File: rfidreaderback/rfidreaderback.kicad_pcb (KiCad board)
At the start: 2 copper layers, 85 x 56 mm, 1 part, among them P1 CONN_13X2

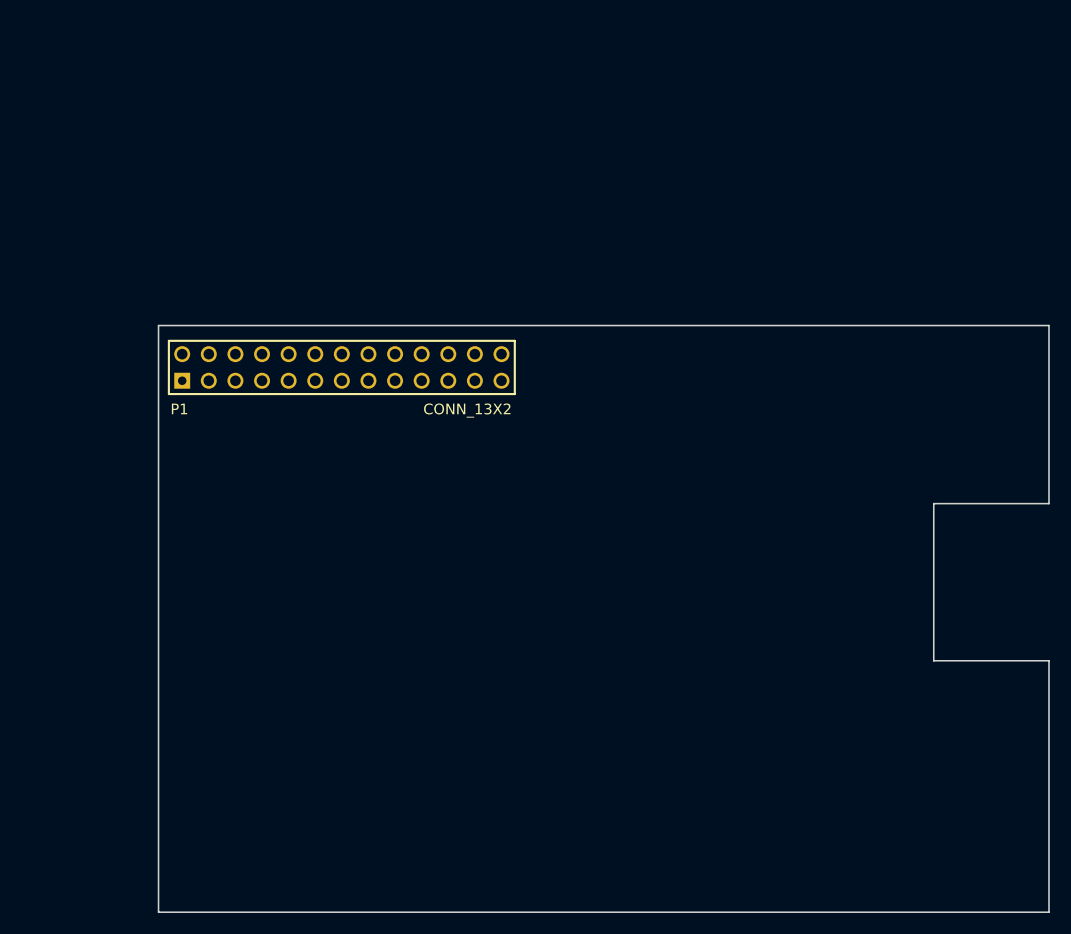
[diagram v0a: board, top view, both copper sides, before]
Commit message: RFID back
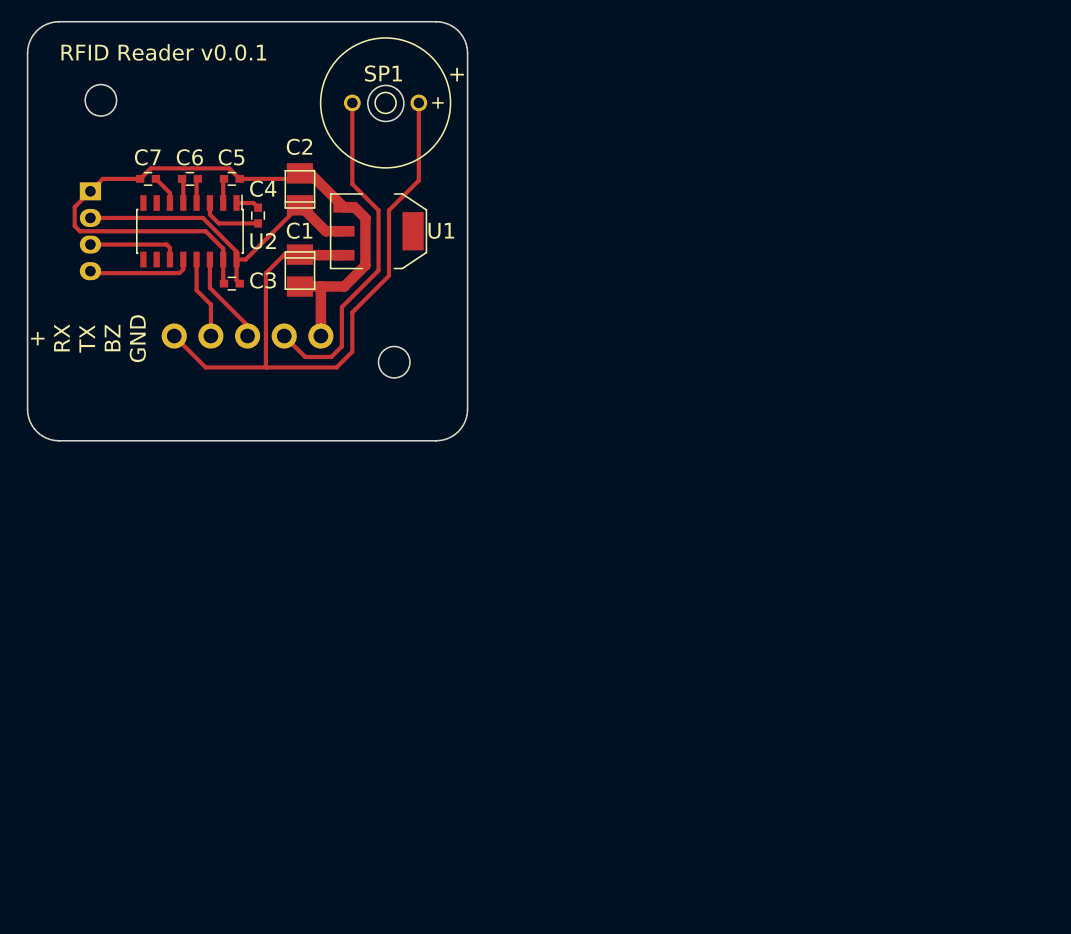
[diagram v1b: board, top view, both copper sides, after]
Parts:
- added C1: 22µ, Capacitors_Tantalum_SMD:TantalC_SizeT_EIA-3528, F.Cu at (157.0, 119.8)
- added C2: 22µ, Capacitors_Tantalum_SMD:TantalC_SizeT_EIA-3528, F.Cu at (157.0, 112.0)
- added C3: 1µ, Capacitors_SMD:C_0603, F.Cu at (150.5, 121.0)
- added C4: 1µ, Capacitors_SMD:C_0603, F.Cu at (153.0, 114.5)
- added C5: 1µ, Capacitors_SMD:C_0603, F.Cu at (150.5, 111.0)
- added C6: 1µ, Capacitors_SMD:C_0603, F.Cu at (146.5, 111.0)
- added C7: 1µ, Capacitors_SMD:C_0603, F.Cu at (142.5, 111.0)
- added P2: PI, pidoor:3_5mm_terminal_1x05, F.Cu at (152.0, 126.0)
- added SP1: MCABI-020-RC, Buzzers_Beepers:MagneticBuzzer_ProSignal_ABT-410-RC, F.Cu at (162.0, 103.8)
- added U1: LD1117S50TR, TO_SOT_Packages_SMD:SOT-223, F.Cu at (164.5, 116.0)
- added U2: ST232BDR, Housings_SOIC:SOIC-16_3.9x9.9mm_Pitch1.27mm, F.Cu at (146.5, 116.0)
- P1: value CONN_13X2 -> READER; footprint pin_array_13x2 -> Socket_Strips:Socket_Strip_Straight_1x04; moved to B.Cu
- moved P1 27.3 mm to (137.0, 116.0), turned to 270 degrees
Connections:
- P1 pad 1: +3.3V -> GND
- P1 pad 3: (no net) -> /TXD
- P1 pad 4: (no net) -> /RXD
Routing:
- net GND: track 0.00 -> 70.4 mm
- net +12V: track 0.00 -> 62.5 mm
- net +5V: track 0.00 -> 32.9 mm
- net /buzzer: track 0.00 -> 32.5 mm
- net /RXD: track 0.00 -> 10.0 mm
- net /TXD: track 0.00 -> 8.83 mm
- net /EIA-TX: track 0.00 -> 8.79 mm
- net /EIA-RX: track 0.00 -> 7.87 mm
- net Net-(C4-Pad2): track 0.00 -> 6.05 mm
- net Net-(C7-Pad2): track 0.00 -> 2.86 mm
- net Net-(C6-Pad2): track 0.00 -> 2.35 mm
- net Net-(C6-Pad1): track 0.00 -> 2.35 mm
- net Net-(C5-Pad2): track 0.00 -> 2.33 mm
- net Net-(C4-Pad1): track 0.00 -> 2.24 mm
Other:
- board size 85 x 56 mm -> 42 x 40 mm
- net class Default: trace_width 0.2 -> 0.4; via_dia 0.9 -> 1
- board text added: "+ RX TX BZ GND"
- board text added: "RFID Reader v0.0.1"
- board text removed: "1/8" JACK OK WITH STD HEADERS !NO TH ABOVE!"
- board text removed: "DOUBLE USB CUTOUT FOR ALL BOARDS"
- board text removed: "RASPBERRY-PI ADDON BOARD VIEW FROM TOP NOTE: P1 SHOULD BE FITTED ON THE REVERSE OF THE BOARD"
- board text removed: "RCA REMOVE WITH STD HEADERS !NO TH ABOVE!"
- board text removed: "RJ45 CUTOUT FOR STD HEADERS !NO TH ABOVE!"
